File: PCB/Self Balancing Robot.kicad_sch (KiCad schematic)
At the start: 27 parts, among them J1 Conn_01x04, J10 Conn_01x02, J2 Conn_01x04, J3 Conn_01x02, J4 -SW, J5 Conn_01x04, J6 Conn_01x04, J7 +SW, J8 +SWLED, J9 -SWLED, U1 GY-521, U2 ESP32-DEVKITC, U5 LM7805_TO220

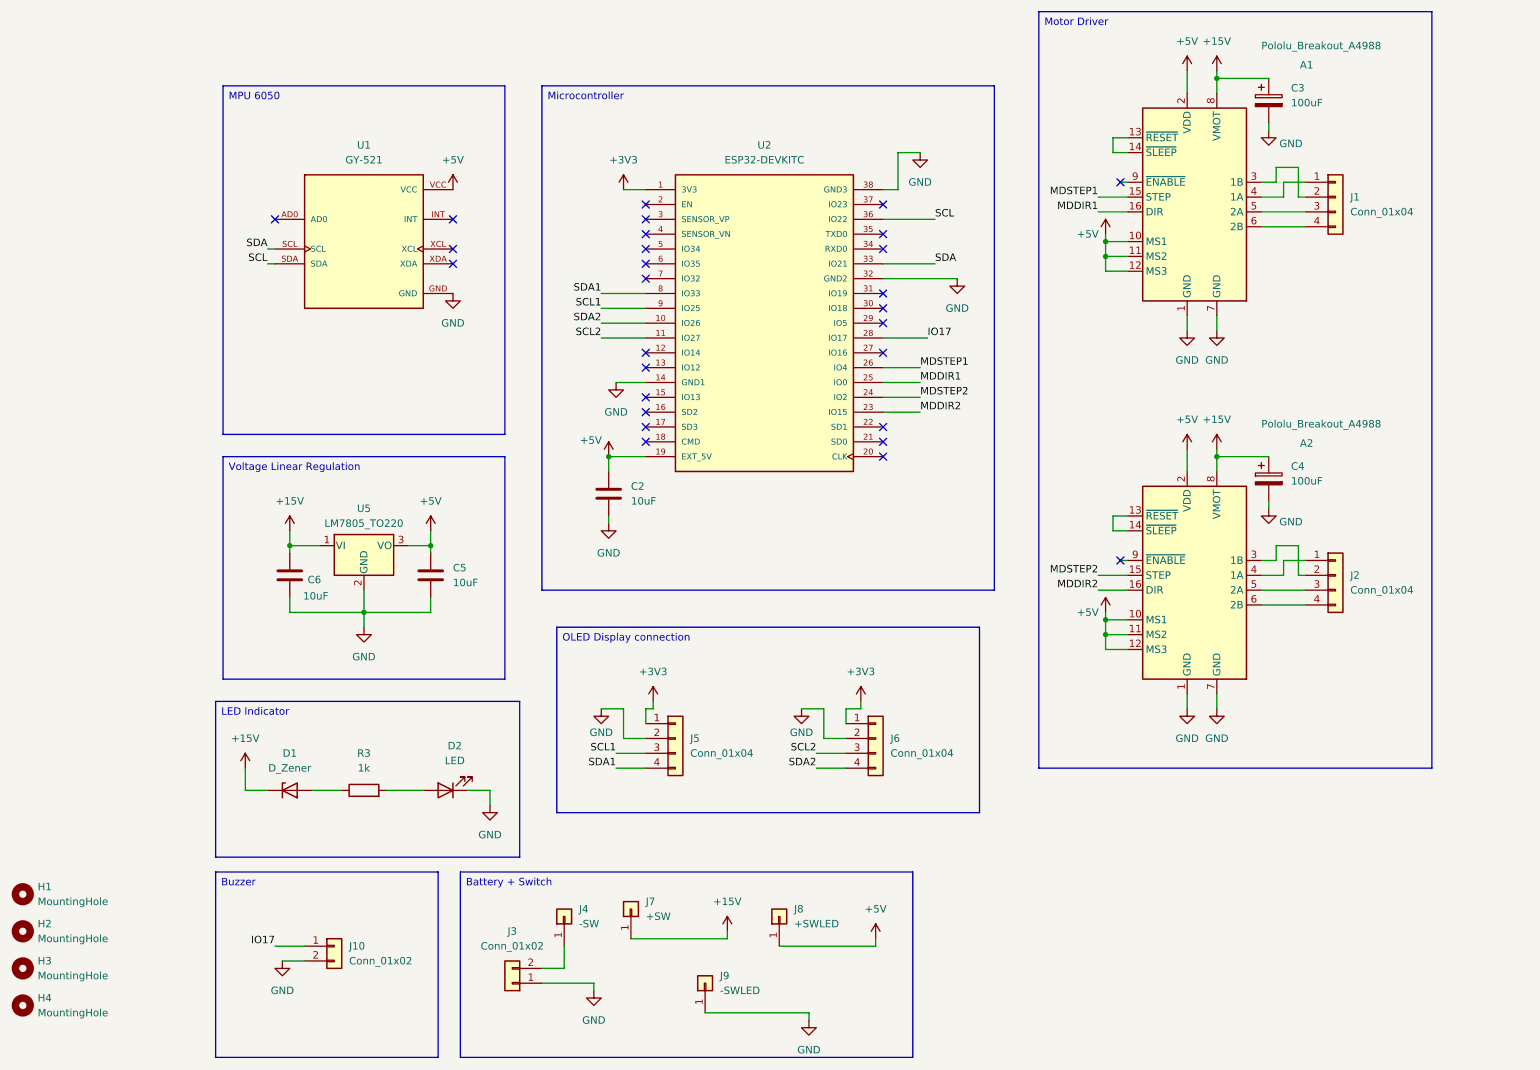
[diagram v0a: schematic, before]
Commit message: Add files via upload
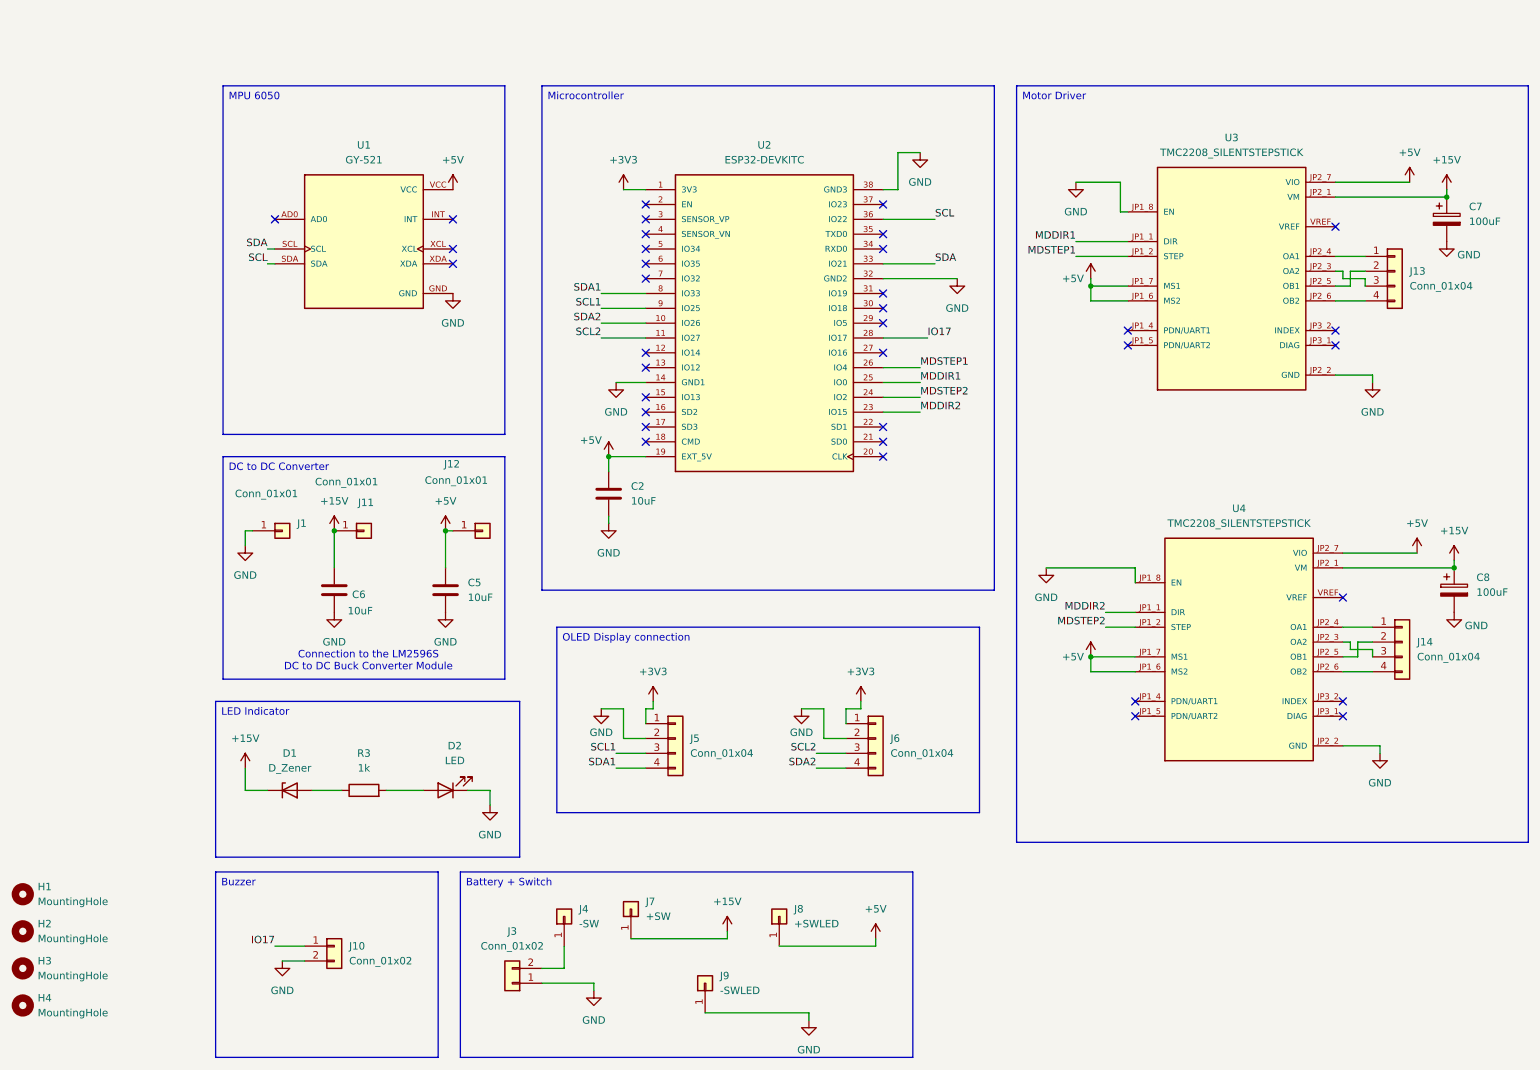
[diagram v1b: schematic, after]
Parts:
- removed A1, A2: Pololu_Breakout_A4988, Module:Pololu_Breakout-16_15.2x20.3mm, symbol Driver_Motor:Pololu_Breakout_A4988
- removed C3, C4: 100uF, Capacitor_THT:CP_Radial_D6.3mm_P2.50mm, symbol Device:C_Polarized
- removed J1, J2: Conn_01x04, Connector_PinHeader_2.54mm:PinHeader_1x04_P2.54mm_Vertical, symbol Connector_Generic:Conn_01x04
- removed U5: LM7805_TO220, Package_TO_SOT_THT:TO-220-3_Vertical, symbol Regulator_Linear:LM7805_TO220
- added C7, C8: 100uF, Capacitor_THT:CP_Radial_D6.3mm_P2.50mm, symbol Device:C_Polarized
- added J1, J11, J12: Conn_01x01, Connector_PinHeader_2.54mm:PinHeader_1x01_P2.54mm_Vertical, symbol Connector_Generic:Conn_01x01
- added J13, J14: Conn_01x04, Connector_PinHeader_2.54mm:PinHeader_1x04_P2.54mm_Vertical, symbol Connector_Generic:Conn_01x04
- added U3, U4: TMC2208_SILENTSTEPSTICK, TMC2208_SILENTSTEPSTICK:MODULE_TMC2208_SILENTSTEPSTICK, symbol TMC2208_SILENTSTEPSTICK:TMC2208_SILENTSTEPSTICK
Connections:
- net +15V: now also C7.1, C8.1, J11.1 (Pin_1), U3.JP2_1 (VM), U4.JP2_1 (VM)
- net +5V: now also J12.1 (Pin_1), U3.JP1_6 (MS2), U3.JP1_7 (MS1), U3.JP2_7 (VIO), U4.JP1_6 (MS2), U4.JP1_7 (MS1), U4.JP2_7 (VIO)
- net GND: now also C7.2, C8.2, J1.1 (Pin_1), U3.JP1_8 (EN), U3.JP2_2 (GND), U3.JP2_8 (GND), U4.JP1_8 (EN), U4.JP2_2 (GND), U4.JP2_8 (GND)
- net MDDIR1: now also U3.JP1_1 (DIR)
- net MDDIR2: now also U4.JP1_1 (DIR)
- net MDSTEP1: now also U3.JP1_2 (STEP)
- net MDSTEP2: now also U4.JP1_2 (STEP)
- new net: J14.1 (Pin_1), U4.JP2_4 (OA1)
- new net: J14.2 (Pin_2), U4.JP2_5 (OB1)
- new net: J14.3 (Pin_3), U4.JP2_3 (OA2)
- new net: J14.4 (Pin_4), U4.JP2_6 (OB2)
- new net: J13.1 (Pin_1), U3.JP2_4 (OA1)
- new net: J13.2 (Pin_2), U3.JP2_5 (OB1)
- new net: J13.3 (Pin_3), U3.JP2_3 (OA2)
- new net: J13.4 (Pin_4), U3.JP2_6 (OB2)
- no-connect marks 28 -> 36
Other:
- note added: "Connection to the LM2596S DC to DC Buck Converter Module"
- title: Qbot - Maritza's Self Balancing Robot -> Qbot - the Self Balancing Robot
- moved on the sheet: C5, C6
